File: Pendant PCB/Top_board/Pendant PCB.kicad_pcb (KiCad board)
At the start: 2 copper layers, 71 x 124 mm, 40 parts, among them J1 Conn_01x20, J2 Conn_01x20, J4 Conn_01x05, J5 Conn_02x02_Odd_Even

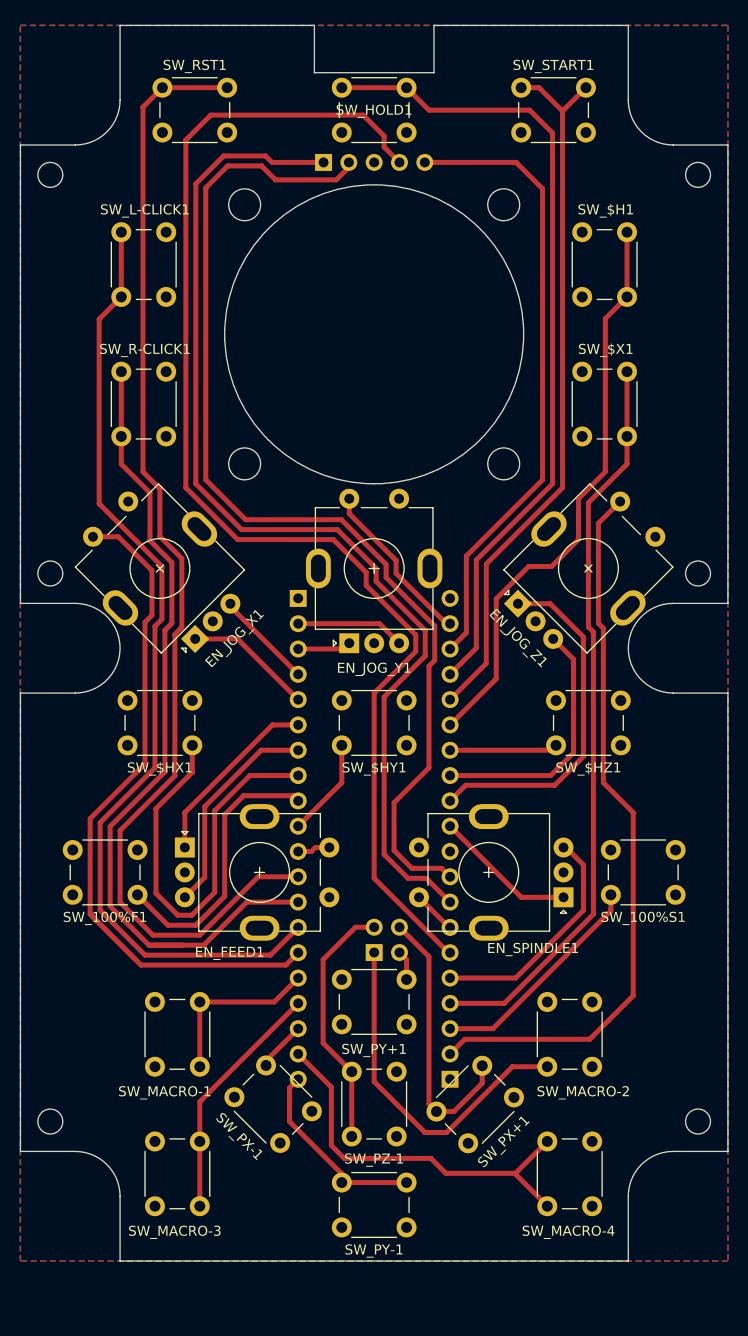
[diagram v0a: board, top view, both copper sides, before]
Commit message: Changes made for 2nd version.
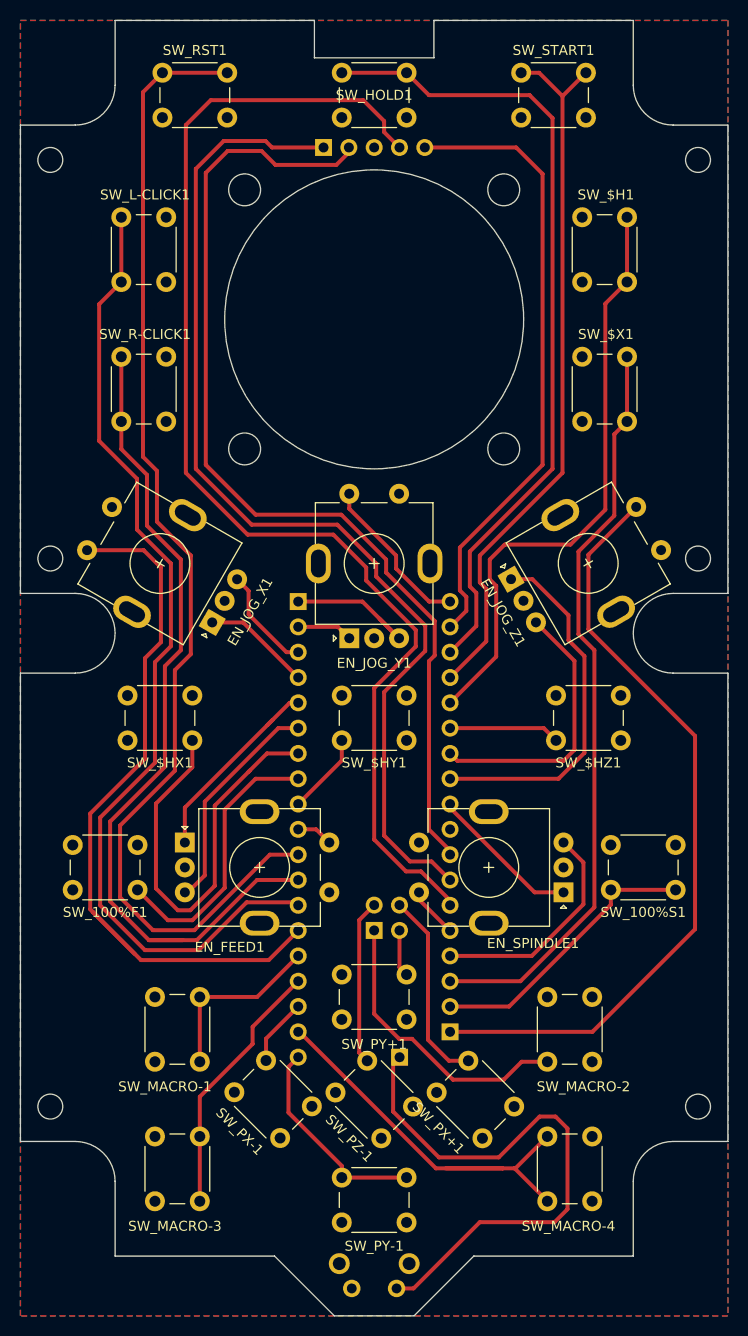
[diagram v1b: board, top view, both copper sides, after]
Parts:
- added J6: Conn_01x01, Connector_PinHeader_2.54mm:PinHeader_1x01_P2.54mm_Vertical, B.Cu at (102.5, 142.6)
- added SW_RST2: SW_Push, Button_Switch_THT:SW_Tactile_SPST_Angled_PTS645Vx39-2LFS, B.Cu at (97.8, 165.8)
- J1: value Conn_01x20 -> Conn_01x19; footprint Connector_PinHeader_2.54mm:PinHeader_1x20_P2.54mm_Vertical -> Connector_PinHeader_2.54mm:PinHeader_1x19_P2.54mm_Vertical
- J2: value Conn_01x20 -> Conn_01x18; footprint Connector_PinHeader_2.54mm:PinHeader_1x20_P2.54mm_Vertical -> Connector_PinHeader_2.54mm:PinHeader_1x18_P2.54mm_Vertical
- moved SW_PX+1 6.02 mm to (109.5, 142.9), turned to 315 degrees
- moved J2 4.76 mm to (107.6, 140.0)
- moved SW_PZ-1 3.15 mm to (99.3, 142.9), turned to 315 degrees
- moved J5 2.22 mm to (100.0, 129.8)
- moved H1 1.50 mm to (67.5, 52.5)
- moved H10 1.50 mm to (113.0, 81.5)
- moved H2 1.50 mm to (132.5, 52.5)
- moved H3 1.50 mm to (67.5, 92.5)
- moved H4 1.50 mm to (132.5, 92.5)
- moved H5 1.50 mm to (67.5, 147.5)
- moved H6 1.50 mm to (132.5, 147.5)
- moved H7 1.50 mm to (87.0, 55.5)
- moved H8 1.50 mm to (113.0, 55.5)
- moved H9 1.50 mm to (87.0, 81.5)
- moved J4 1.50 mm to (94.9, 51.2)
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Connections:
- net /A2 renamed /A1
- EN_SPINDLE1 pad S2: /39 -> /40
- J1 pad 1: GND -> /27
- J1 pad 10: /7 -> /8
- J1 pad 11: /8 -> /9
- J1 pad 12: /9 -> /10
- J1 pad 13: /10 -> /11
- J1 pad 14: /11 -> /12
- J1 pad 15: /12 -> /13
- J1 pad 16: /13 -> /14
- J1 pad 17: /14 -> /15
- J1 pad 18: /15 -> /16
- J1 pad 19: /16 -> /17
- J1 pad 2: /27 -> /0
- J1 pad 3: /0 -> /1
- J1 pad 4: /1 -> /2
- J1 pad 5: /2 -> /3
- J1 pad 6: /3 -> /4
- J1 pad 7: /4 -> /5
- J1 pad 8: /5 -> /6
- J1 pad 9: /6 -> /7
- J2 pad 1: /45 -> /44
- J2 pad 10: GND -> /18
- J2 pad 11: /18 -> /19
- J2 pad 12: /19 -> /20
- J2 pad 13: /20 -> /21
- J2 pad 14: /21 -> /22
- J2 pad 15: /22 -> /23
- J2 pad 16: /23 -> /24
- J2 pad 17: /24 -> /25
- J2 pad 18: /25 -> /26
- J2 pad 2: /44 -> /43
- J2 pad 3: /43 -> /42
- J2 pad 4: /42 -> /41
- J2 pad 5: /41 -> /40
- J2 pad 7: /39 -> /A0
- J2 pad 8: /A0 -> +5VA
- J2 pad 9: +5VA -> GND
- SW_PZ-1 pad 1: GND -> /32
- SW_PZ-1 pad 2: /32 -> GND
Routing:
- net /RS: track 0.00 -> 55.9 mm
- net /32: track 25.4 -> 16.6 mm
- net /28: track 27.6 -> 19.6 mm
- net +5VA: track 106.9 -> 101.0 mm
- net /33: track 35.2 -> 29.2 mm
- net /43: track 22.6 -> 28.4 mm
- net /40: track 0.00 -> 5.13 mm
- net /44: track 72.8 -> 77.6 mm
- net /39: track 4.37 -> 0.00 mm
- net /27: track 10.9 -> 14.4 mm
- net /A1: track 126.8 -> 123.8 mm
- net /16: track 39.4 -> 42.4 mm
- net /11: track 97.0 -> 99.7 mm
- net /17: track 19.4 -> 22.1 mm
- net /9: track 114.9 -> 117.4 mm
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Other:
- board size 71 x 124 mm -> 71 x 130 mm
- net class Default: clearance 0.47 -> 0.37; trace_width 0.3 -> 0.4
- rule trace_clearance: 0.47 -> 0.37
